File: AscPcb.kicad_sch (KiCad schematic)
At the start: 92 parts, among them J1 12402012E212A, J10 Conn_01x02_Pin, J11 Conn_01x02_Pin, J12 Conn_01x02_Pin, J13 Conn_01x02_Pin, J14 Conn_01x02_Pin, J15 Conn_01x02_Pin, J16 Conn_01x02_Pin, J2 B2B-PH-K-S(LF)(SN), J3 Screw_Terminal_01x02, J4 Screw_Terminal_01x02, J5 Conn_01x15_Pin, J6 Conn_01x06_Pin, J7 Conn_01x02_Pin, J8 Conn_01x02_Pin, J9 Conn_01x03_Pin, Q1 Q_NMOS_DGS, Q2 BC817, Q3 BC817, SW1 TL3305AF260QG, SW2 TL3305AF260QG, U1 BQ24040DSQR, U2 TLV75801PDRVR, U3 AP62300TWU, U4 LTC3625EDE_PBF, U5 ESP32-C3-WROOM-02-N4, U6 CP2102N-A02-GQFN24R, U7 BMI270, U8 74LVC1G07

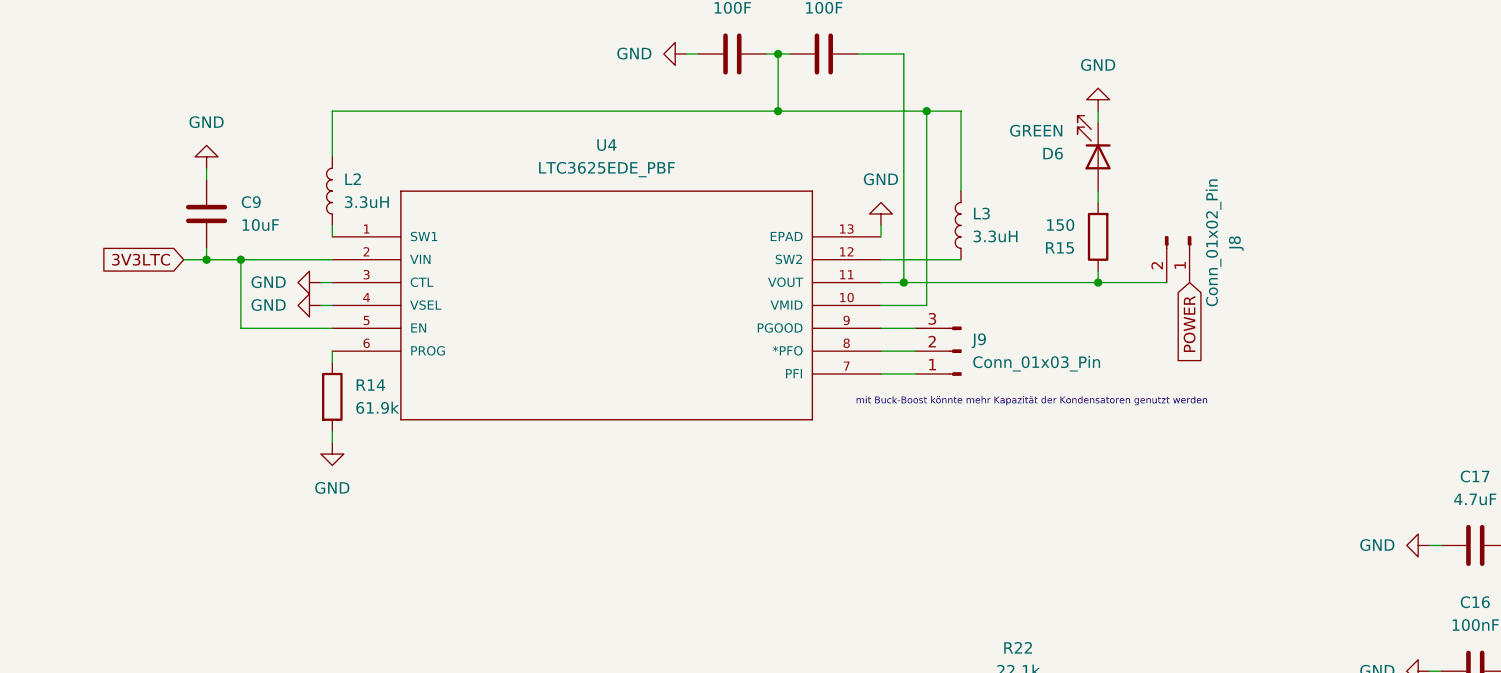
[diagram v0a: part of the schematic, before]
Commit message: double checked everything in schematic
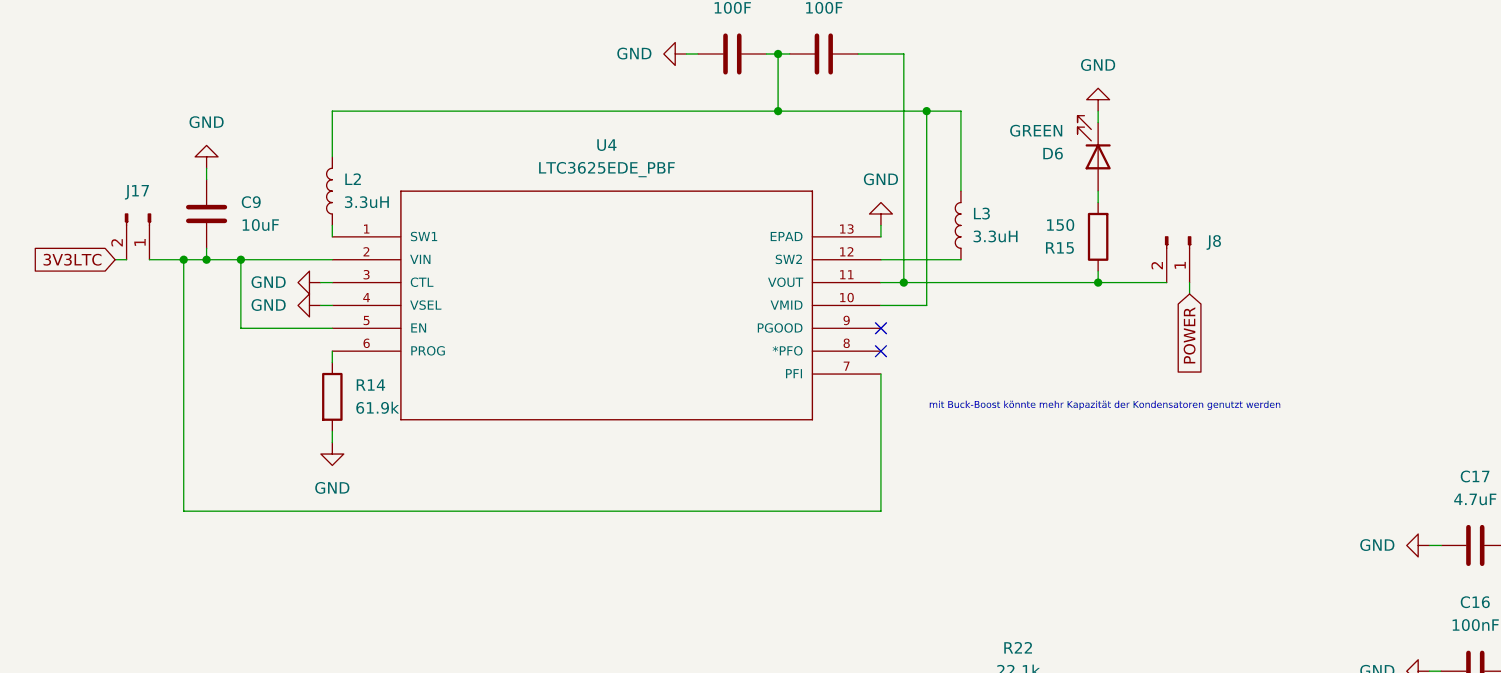
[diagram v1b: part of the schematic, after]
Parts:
- removed J9: Conn_01x03_Pin, Connector_PinHeader_2.54mm:PinHeader_1x03_P2.54mm_Vertical, symbol Connector:Conn_01x03_Pin
- added J17: Conn_01x02_Pin, Connector_PinHeader_2.54mm:PinHeader_1x02_P2.54mm_Vertical, symbol Connector:Conn_01x02_Pin
- L1: footprint Inductor_SMD:L_0805_2012Metric -> DR73-3R3-R:DR73-3R3-R_EAT; MPN MLZ2012M3R3ATD69 -> DR73-3R3-R
- L2, L3: MPN DR73-3R3-R -> DR73-3R3-R
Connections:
- net 3V3LTC: now also J17.2 (Pin_2); no longer C9.2, U4.2 (VIN), U4.5 (EN)
- net at U4.7 (PFI): now also C9.2, U4.2 (VIN), U4.5 (EN), J17.1 (Pin_1)
- no-connect marks 18 -> 20
